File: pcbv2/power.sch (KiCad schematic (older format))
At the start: 13 parts, among them SW4 SW_SPDT, U2 AMS1117-3.3, U4 TPS610986DSET, U6 PMPB15XP,115

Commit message: feat(pcbv2): add part numbers to schematics
mostly LCSC / Digikey. Some components still missing, will
add them soon.
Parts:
- U6: Description (none) -> Trans MOSFET P-CH 12V 8.2A 6-Pin DFN-MD EP T/R; Field4 UDFN-6 Nexperia USA -> (none); Field5 Nexperia USA -> (none); Field6 None -> (none); Field7 Unavailable -> (none); Field8 Trans MOSFET P-CH 12V 8.2A 6-Pin DFN-MD EP T/R -> (none); LCSC Part (none) -> C294617
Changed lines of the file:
@@
 F 1 "PMPB15XP,115" H 4700 4700 50  0000 L CNN
 F 2 "PMPB15XP_115:MOSFET_PMPB55ENEAX" H 5350 5050 50  0001 L BNN
-F 3 "PMPB15XP,115" H 5350 5050 50  0001 L BNN
-F 4 "UDFN-6 Nexperia USA" H 5350 5050 50  0001 L BNN "Field4"
-F 5 "Nexperia USA" H 5350 5050 50  0001 L BNN "Field5"
-F 6 "None" H 5350 5050 50  0001 L BNN "Field6"
-F 7 "Unavailable" H 5350 5050 50  0001 L BNN "Field7"
-F 8 "Trans MOSFET P-CH 12V 8.2A 6-Pin DFN-MD EP T/R" H 5350 5050 50  0001 L BNN "Field8"
+F 3 "~" H 5350 5050 50  0001 L BNN
+F 4 "Trans MOSFET P-CH 12V 8.2A 6-Pin DFN-MD EP T/R" H 5350 5050 50  0001 L BNN "Description"
+F 5 "C294617" H 5350 5050 50  0001 C CNN "LCSC Part"
 	1    5350 5050
 	1    0    0    -1

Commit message: feat(pcbv2): add BOM part numbers
most parts there there, still missing a few
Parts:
- C12: LCSC Part (none) -> C27279; Vendor (none) -> TLJA107M006R0800
- L2: LCSC Part (none) -> C307785; Vendor (none) -> NLCV32T-4R7M-PFR
- R14: LCSC Part (none) -> C23151; Vendor (none) -> 0603WAF3900T5E
- SW4: Digikey Part (none) -> CKN9560-ND; Vendor (none) -> OS102011MA1QS1
- U2: LCSC Part (none) -> C6186
- U4: Digikey Part (none) -> 296-44974-1-ND; LCSC Part (none) -> C73820
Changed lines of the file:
@@
 F 2 "SON50P150X150X80-6N:SON50P150X150X80-6N" H 7400 3450 50  0001 C CNN
 F 3 "" H 7400 3450 50  0001 C CNN
+F 4 "296-44974-1-ND" H 7500 3600 50  0001 C CNN "Digikey Part"
+F 5 "C73820" H 7500 3600 50  0001 C CNN "LCSC Part"
 	1    7500 3600
 	1    0    0    -1
@@
 F 2 "Package_TO_SOT_SMD:SOT-223-3_TabPin2" H 4550 3700 50  0001 C CNN
 F 3 "http://www.advanced-monolithic.com/pdf/ds1117.pdf" H 4650 3250 50  0001 C CNN
+F 4 "C6186" H 4550 3500 50  0001 C CNN "LCSC Part"
 	1    4550 3500
 	1    0    0    -1
@@
 F 2 "Inductor_SMD:L_1210_3225Metric" H 6750 3600 50  0001 C CNN
 F 3 "~" H 6750 3600 50  0001 C CNN
+F 4 "C307785" H 6750 3600 50  0001 C CNN "LCSC Part"
+F 5 "NLCV32T-4R7M-PFR" H 6750 3600 50  0001 C CNN "Vendor"
 	1    6750 3600
 	1    0    0    -1
@@
 F 2 "Resistor_SMD:R_0603_1608Metric" V 6230 3750 50  0001 C CNN
 F 3 "~" H 6300 3750 50  0001 C CNN
+F 4 "C23151" H 6300 3750 50  0001 C CNN "LCSC Part"
+F 5 "0603WAF3900T5E" H 6300 3750 50  0001 C CNN "Vendor"
 	1    6300 3750
 	1    0    0    -1
@@
 F 2 "Button_Switch_THT:SW_CuK_OS102011MA1QN1_SPDT_Angled" H 5600 3600 50  0001 C CNN
 F 3 "" H 5600 3600 50  0001 C CNN
+F 4 "CKN9560-ND" H 5600 3600 50  0001 C CNN "Digikey Part"
+F 5 "OS102011MA1QS1" H 5600 3600 50  0001 C CNN "Vendor"
 	1    5600 3600
 	-1   0    0    1
@@
 F 2 "Capacitor_Tantalum_SMD:CP_EIA-3216-18_Kemet-A" H 6750 2950 50  0001 C CNN
 F 3 "~" H 6750 2950 50  0001 C CNN
+F 4 "C27279" H 6750 2950 50  0001 C CNN "LCSC Part"
+F 5 "TLJA107M006R0800" H 6750 2950 50  0001 C CNN "Vendor"
 	1    6750 2950
 	-1   0    0    1

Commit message: Added battery holders BOM data
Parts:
- BT1: footprint AA_battery_clip:BK-53_MPD_AAClip -> bcaaapc:bcaaapc; Digikey Part (none) -> BCAAAPC-ND
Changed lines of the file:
@@
 EESchema Schematic File Version 4
 LIBS:badge2-cache
-EELAYER 30 0
+EELAYER 26 0
 EELAYER END
 $Descr A4 11693 8268
@@
 F 0 "BT1" H 3768 4946 50  0000 L CNN
 F 1 "Battery_Cell" H 3768 4855 50  0000 L CNN
-F 2 "AA_battery_clip:BK-53_MPD_AAClip" V 3650 4910 50  0001 C CNN
-F 3 "~" V 3650 4910 50  0001 C CNN
+F 2 "bcaaapc:bcaaapc" V 3650 4910 50  0001 C CNN
+F 3 "http://www.memoryprotectiondevices.com/datasheets/BCAAAPC-datasheet.pdf" V 3650 4910 50  0001 C CNN
+F 4 "BCAAAPC-ND" H 3650 4850 50  0001 C CNN "Digikey Part"
 	1    3650 4850
 	0    1    1    0

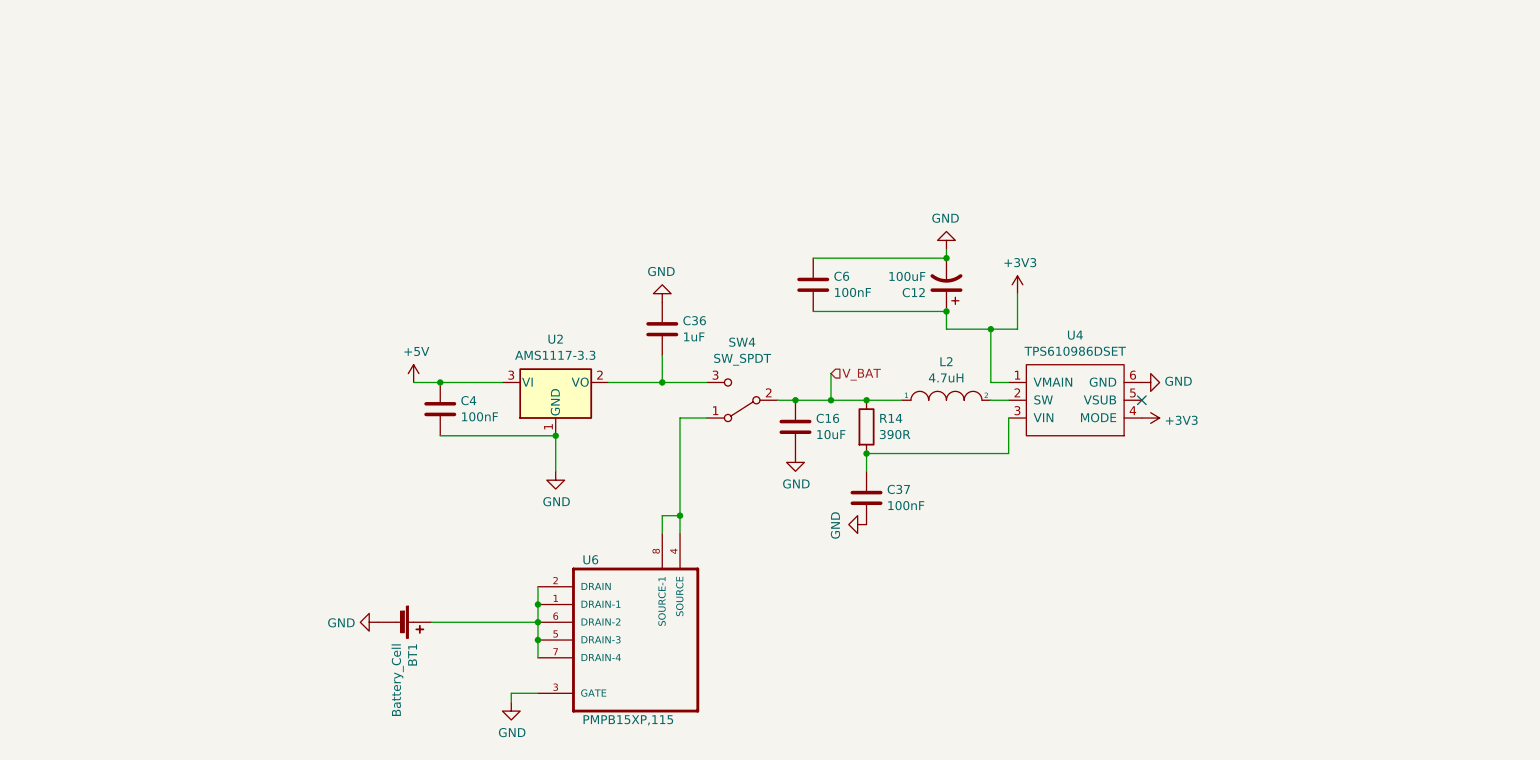
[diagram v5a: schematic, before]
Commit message: fix(pcbv2): remove AMS1117-3.3 regulator
We already have RT9013-33GB that does the same.
This also fixes an issue where the power switch would not be able to cut USB/LiPo power.
Also move LiPo circuit into power schematic.
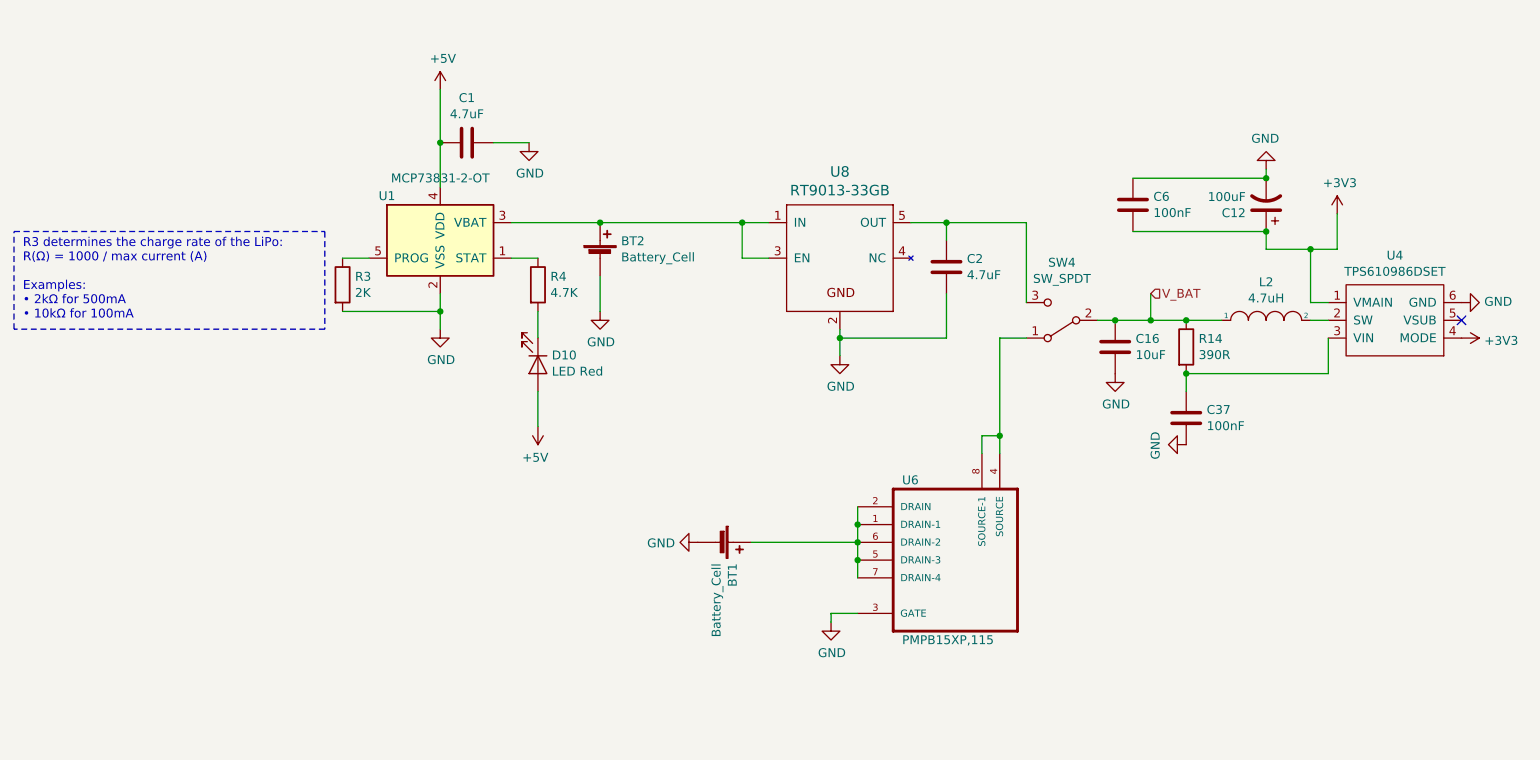
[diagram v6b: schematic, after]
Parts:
- removed C36: 1uF, Capacitor_SMD:C_0603_1608Metric, symbol Device:C
- removed C4: 100nF, Capacitor_SMD:C_0603_1608Metric, symbol Device:C
- removed U2: AMS1117-3.3, Package_TO_SOT_SMD:SOT-223-3_TabPin2, symbol Regulator_Linear:AMS1117-3.3
- added BT2: Battery_Cell, jst:JST_PH_B2B-PH-K_02x2.00mm_Straight, symbol Device:Battery_Cell
- added C1, C2: 4.7uF, Capacitor_SMD:C_0603_1608Metric, symbol Device:C
- added D10: LED Red, LED_SMD:LED_0603_1608Metric, symbol Device:LED
- added R3: 2K, Resistor_SMD:R_0603_1608Metric, symbol Device:R
- added R4: 4.7K, Resistor_SMD:R_0603_1608Metric, symbol Device:R
- added U1: MCP73831-2-OT, Package_TO_SOT_SMD:SOT-23-5, symbol Battery_Management:MCP73831-2-OT
- added U8: RT9013-33GB, Package_TO_SOT_SMD:SOT-23-5, symbol RT9013:RT9013-XXXB
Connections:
- net +5V: now also C1.2, D10.2 (A), U1.4 (VDD)
- net GND: now also BT2.2 (-), C1.1, C2.2, R3.2, U1.2 (VSS), U8.2 (GND)
- net at SW4.3 (C): now also C2.1, U8.5 (OUT)
- new net: R4.1, U1.1 (STAT)
- new net: BT2.1 (+), U1.3 (VBAT), U8.1 (IN), U8.3 (EN)
- new net: R3.1, U1.5 (PROG)
- new net: D10.1 (K), R4.2
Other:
- note added: "R3 determines the charge rate of the LiPo:\nR(Ω) = 1000 / max current (A) \n\nExamples:\n• 2kΩ for 500mA\n• 10kΩ for 100mA"
- moved on the sheet: BT1, C12, C16, C37, C6, L2, R14, SW4, U4, U6

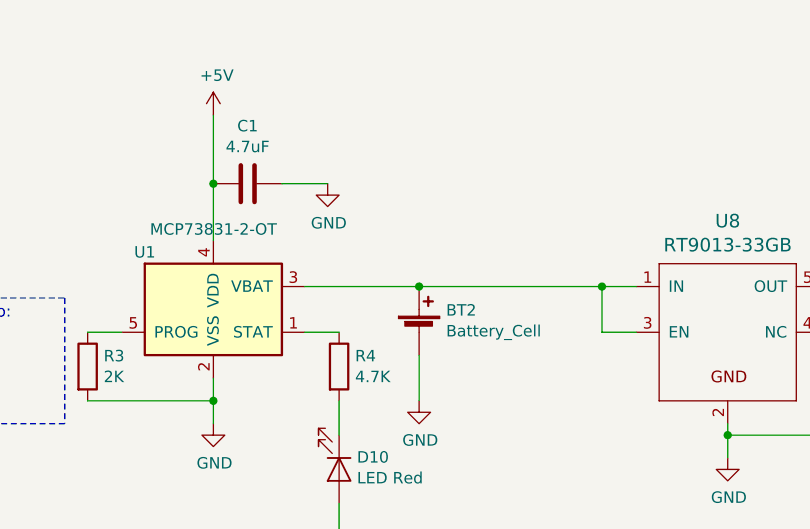
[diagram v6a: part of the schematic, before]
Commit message: feat(pcbv2): improve LiPo charging circuit
Add a transistor (Q3), that cuts the power from the LiPo when USB is connected,
allowing us to separate the battery from the rest of the circuit
while it's being charged.
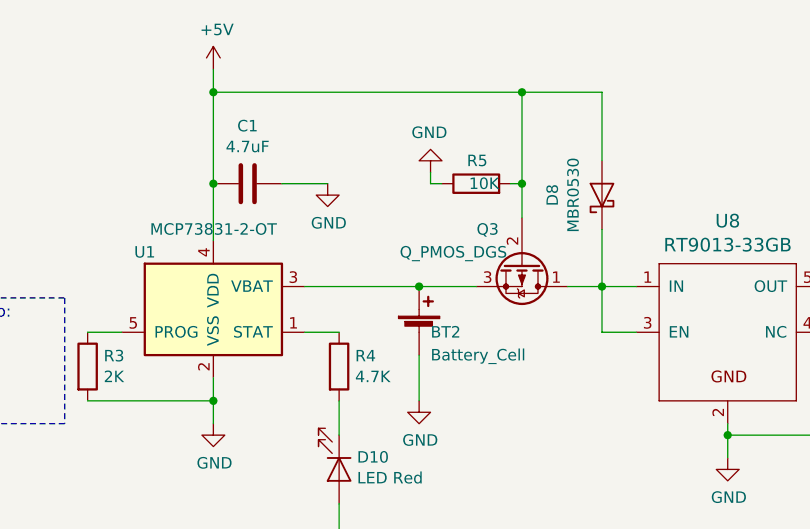
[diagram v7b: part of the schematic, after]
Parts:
- added D8: MBR0530, Diode_SMD:D_SOD-123, symbol Device:D_Schottky
- added Q3: Q_PMOS_DGS, Package_TO_SOT_SMD:SOT-23, symbol Device:Q_PMOS_DGS
- added R5: 10K, Resistor_SMD:R_0603_1608Metric, symbol Device:R
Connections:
- net +5V: now also D8.2 (A), Q3.2 (G), R5.2
- net GND: now also R5.1
- net at BT2.1 (+), U1.3 (VBAT): now also Q3.3 (S); no longer U8.1 (IN), U8.3 (EN)
- new net: D8.1 (K), Q3.1 (D), U8.1 (IN), U8.3 (EN)
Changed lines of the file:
@@
 L power:+5V #PWR0109
 U 1 1 5D9D5A8E
-P 3900 1850
-F 0 "#PWR0109" H 3900 1700 50  0001 C CNN
-F 1 "+5V" H 3915 2023 50  0000 C CNN
-F 2 "" H 3900 1850 50  0001 C CNN
-F 3 "" H 3900 1850 50  0001 C CNN
-	1    3900 1850
-	1    0    0    -1
-$EndComp
-Wire Wire Line
-	3900 1850 3900 2150
+P 3900 1650
+F 0 "#PWR0109" H 3900 1500 50  0001 C CNN
+F 1 "+5V" H 3915 1823 50  0000 C CNN
+F 2 "" H 3900 1650 50  0001 C CNN
+F 3 "" H 3900 1650 50  0001 C CNN
+	1    3900 1650
+	1    0    0    -1
+$EndComp
 Wire Wire Line
 	4300 2600 4800 2600
@@
 U 1 1 5D9D64A0
 P 4800 2800
-F 0 "BT2" H 4918 2896 50  0000 L CNN
-F 1 "Battery_Cell" H 4918 2805 50  0000 L CNN
+F 0 "BT2" H 4850 2800 50  0000 L CNN
+F 1 "Battery_Cell" H 4850 2700 50  0000 L CNN
 F 2 "jst:JST_PH_B2B-PH-K_02x2.00mm_Straight" V 4800 2860 50  0001 C CNN
 F 3 "http://www.jst-mfg.com/product/pdf/eng/ePH.pdf" V 4800 2860 50  0001 C CNN
@@
 	6750 3250 6150 3250
 Wire Wire Line
-	4800 2600 5600 2600
+	4800 2600 5050 2600
 Connection ~ 6150 3250
 Wire Wire Line
@@
 	7200 2600 6750 2600
 Connection ~ 6750 2600
+$Comp
+L Device:Q_PMOS_DGS Q3
+U 1 1 5DBF0489
+P 5250 2500
+F 0 "Q3" V 5100 2350 50  0000 C CNN
+F 1 "Q_PMOS_DGS" V 5200 2200 50  0000 C CNN
+F 2 "Package_TO_SOT_SMD:SOT-23" H 5450 2600 50  0001 C CNN
+F 3 "~" H 5250 2500 50  0001 C CNN
+F 4 "C15127" V 5250 2500 50  0001 C CNN "LCSC Part"
+F 5 "AO3401A" V 5250 2500 50  0001 C CNN "Vendor"
+	1    5250 2500
+	0    1    1    0
+$EndComp
+Wire Wire Line
+	5450 2600 5600 2600
+Wire Wire Line
+	3900 1650 3900 1750
+Wire Wire Line
+	5250 2300 5250 2150
+Connection ~ 3900 1750
+Wire Wire Line
+	3900 1750 3900 2150
+$Comp
+L Device:R R?
+U 1 1 5DBFE530
+P 5050 2150
+AR Path="/5DBFE530" Ref="R?"  Part="1"
+AR Path="/5C4AA0D1/5DBFE530" Ref="R5"  Part="1"
+F 0 "R5" V 5150 2100 50  0000 L CNN
+F 1 "10K" V 5050 2050 50  0000 L CNN
+F 2 "Resistor_SMD:R_0603_1608Metric" V 4980 2150 50  0001 C CNN
+F 3 "~" H 5050 2150 50  0001 C CNN
+F 4 "C25804" H 5050 2150 50  0001 C CNN "LCSC Part"
+F 5 "0603WAF1002T5E" H 5050 2150 50  0001 C CNN "Vendor"
+	1    5050 2150
+	0    -1   -1   0
+$EndComp
+Connection ~ 5250 2150
+Wire Wire Line
+	5250 2150 5250 1750
+$Comp
+L power:GND #PWR0113
+U 1 1 5DC02497
+P 4850 2100
+F 0 "#PWR0113" H 4850 1850 50  0001 C CNN
+F 1 "GND" H 4855 1927 50  0000 C CNN
+F 2 "" H 4850 2100 50  0001 C CNN
+F 3 "" H 4850 2100 50  0001 C CNN
+	1    4850 2100
+	-1   0    0    1
+$EndComp
+Wire Wire Line
+	4850 2150 4850 2100
+Wire Wire Line
+	3900 1750 5250 1750
+Connection ~ 5250 1750
+Wire Wire Line
+	5250 1750 5600 1750
+Wire Wire Line
+	5600 1750 5600 2050
+Wire Wire Line
+	5600 2350 5600 2600
+Wire Wire Line
+	4900 2150 4850 2150
+Wire Wire Line
+	5200 2150 5250 2150
+$Comp
+L Device:D_Schottky D8
+U 1 1 5DC18B11
+P 5600 2200
+F 0 "D8" H 5600 2416 50  0000 C CNN
+F 1 "MBR0530" H 5600 2325 50  0000 C CNN
+F 2 "Diode_SMD:D_SOD-123" H 5600 2200 50  0001 C CNN
+F 3 "~" H 5600 2200 50  0001 C CNN
+F 4 "C77336" H 5600 2200 50  0001 C CNN "LCSC Part"
+	1    5600 2200
+	0    -1   -1   0
+$EndComp
 $EndSCHEMATC

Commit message: fix(pcbv2): Q3 mosfet orientation
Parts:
- Q3: symbol Device:Q_PMOS_DGS -> Device:Q_PMOS_GSD
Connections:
- net +5V: now also Q3.1 (G); no longer Q3.2 (G)
- net at D8.1 (K), U8.1 (IN), U8.3 (EN): now also Q3.2 (S); no longer Q3.1 (D)
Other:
- moved on the sheet: BT2, D8, Q3, R5
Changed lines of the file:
@@
 	1    0    0    -1
 $EndComp
-Wire Wire Line
-	4300 2600 4800 2600
 $Comp
 L Device:Battery_Cell BT2
 U 1 1 5D9D64A0
-P 4800 2800
-F 0 "BT2" H 4850 2800 50  0000 L CNN
-F 1 "Battery_Cell" H 4850 2700 50  0000 L CNN
-F 2 "jst:JST_PH_B2B-PH-K_02x2.00mm_Straight" V 4800 2860 50  0001 C CNN
-F 3 "http://www.jst-mfg.com/product/pdf/eng/ePH.pdf" V 4800 2860 50  0001 C CNN
-F 4 "B2B-PH-K-S(LF)(SN)" H 4800 2800 50  0001 C CNN "Digikey Part"
-	1    4800 2800
-	1    0    0    -1
-$EndComp
-Wire Wire Line
-	4800 2900 4800 3100
+P 4850 2400
+F 0 "BT2" H 4850 2400 50  0000 L CNN
+F 1 "Battery_Cell" H 4650 2300 50  0000 L CNN
+F 2 "jst:JST_PH_B2B-PH-K_02x2.00mm_Straight" V 4850 2460 50  0001 C CNN
+F 3 "http://www.jst-mfg.com/product/pdf/eng/ePH.pdf" V 4850 2460 50  0001 C CNN
+F 4 "B2B-PH-K-S(LF)(SN)" H 4850 2400 50  0001 C CNN "Digikey Part"
+	1    4850 2400
+	-1   0    0    1
+$EndComp
 Connection ~ 3900 3100
 Wire Wire Line
@@
 $EndComp
 Wire Wire Line
-	4450 3550 4450 3750
+	4450 3550 4450 3650
 $Comp
 L RT9013:RT9013-XXXB U8
@@
 	1    0    0    -1
 $EndComp
-Connection ~ 4800 2600
 Wire Wire Line
 	5600 2600 5600 2800
@@
 Wire Wire Line
 	6750 3250 6150 3250
-Wire Wire Line
-	4800 2600 5050 2600
 Connection ~ 6150 3250
 Wire Wire Line
@@
 	7200 2600 6750 2600
 Connection ~ 6750 2600
-$Comp
-L Device:Q_PMOS_DGS Q3
-U 1 1 5DBF0489
-P 5250 2500
-F 0 "Q3" V 5100 2350 50  0000 C CNN
-F 1 "Q_PMOS_DGS" V 5200 2200 50  0000 C CNN
-F 2 "Package_TO_SOT_SMD:SOT-23" H 5450 2600 50  0001 C CNN
-F 3 "~" H 5250 2500 50  0001 C CNN
-F 4 "C15127" V 5250 2500 50  0001 C CNN "LCSC Part"
-F 5 "AO3401A" V 5250 2500 50  0001 C CNN "Vendor"
-	1    5250 2500
-	0    1    1    0
-$EndComp
 Wire Wire Line
 	5450 2600 5600 2600
-Wire Wire Line
-	3900 1650 3900 1750
-Wire Wire Line
-	5250 2300 5250 2150
-Connection ~ 3900 1750
-Wire Wire Line
-	3900 1750 3900 2150
 $Comp
 L Device:R R?
 U 1 1 5DBFE530
-P 5050 2150
+P 5050 3000
 AR Path="/5DBFE530" Ref="R?"  Part="1"
 AR Path="/5C4AA0D1/5DBFE530" Ref="R5"  Part="1"
-F 0 "R5" V 5150 2100 50  0000 L CNN
-F 1 "10K" V 5050 2050 50  0000 L CNN
-F 2 "Resistor_SMD:R_0603_1608Metric" V 4980 2150 50  0001 C CNN
-F 3 "~" H 5050 2150 50  0001 C CNN
-F 4 "C25804" H 5050 2150 50  0001 C CNN "LCSC Part"
-F 5 "0603WAF1002T5E" H 5050 2150 50  0001 C CNN "Vendor"
-	1    5050 2150
+F 0 "R5" V 5150 2950 50  0000 L CNN
+F 1 "10K" V 5050 2900 50  0000 L CNN
+F 2 "Resistor_SMD:R_0603_1608Metric" V 4980 3000 50  0001 C CNN
+F 3 "~" H 5050 3000 50  0001 C CNN
+F 4 "C25804" H 5050 3000 50  0001 C CNN "LCSC Part"
+F 5 "0603WAF1002T5E" H 5050 3000 50  0001 C CNN "Vendor"
+	1    5050 3000
 	0    -1   -1   0
 $EndComp
-Connection ~ 5250 2150
-Wire Wire Line
-	5250 2150 5250 1750
 $Comp
 L power:GND #PWR0113
 U 1 1 5DC02497
-P 4850 2100
-F 0 "#PWR0113" H 4850 1850 50  0001 C CNN
-F 1 "GND" H 4855 1927 50  0000 C CNN
-F 2 "" H 4850 2100 50  0001 C CNN
-F 3 "" H 4850 2100 50  0001 C CNN
-	1    4850 2100
+P 4850 2050
+F 0 "#PWR0113" H 4850 1800 50  0001 C CNN
+F 1 "GND" H 4855 1877 50  0000 C CNN
+F 2 "" H 4850 2050 50  0001 C CNN
+F 3 "" H 4850 2050 50  0001 C CNN
+	1    4850 2050
 	-1   0    0    1
 $EndComp
 Wire Wire Line
-	4850 2150 4850 2100
-Wire Wire Line
-	3900 1750 5250 1750
-Connection ~ 5250 1750
-Wire Wire Line
-	5250 1750 5600 1750
-Wire Wire Line
-	5600 1750 5600 2050
-Wire Wire Line
-	5600 2350 5600 2600
-Wire Wire Line
-	4900 2150 4850 2150
-Wire Wire Line
-	5200 2150 5250 2150
+	5200 3000 5250 3000
+$Comp
+L Device:Q_PMOS_GSD Q3
+U 1 1 5DBF0489
+P 5250 2700
+F 0 "Q3" V 5600 2700 50  0000 C CNN
+F 1 "Q_PMOS_DGS" V 5500 2700 50  0000 C CNN
+F 2 "Package_TO_SOT_SMD:SOT-23" H 5450 2800 50  0001 C CNN
+F 3 "~" H 5250 2700 50  0001 C CNN
+F 4 "C15127" V 5250 2700 50  0001 C CNN "LCSC Part"
+F 5 "AO3401A" V 5250 2700 50  0001 C CNN "Vendor"
+	1    5250 2700
+	0    -1   -1   0
+$EndComp
+Wire Wire Line
+	4450 3650 5250 3650
+Wire Wire Line
+	5250 3650 5250 3250
+Connection ~ 4450 3650
+Wire Wire Line
+	4450 3650 4450 3750
+Wire Wire Line
+	5600 2800 5600 2950
+Connection ~ 5600 2800
+Wire Wire Line
+	5600 3250 5250 3250
+Connection ~ 5250 3250
+Wire Wire Line
+	5250 3250 5250 3000
+Wire Wire Line
+	3900 1650 3900 2150
+Wire Wire Line
+	4300 2600 4850 2600
+Connection ~ 4850 2600
+Wire Wire Line
+	4850 2600 5050 2600
+Connection ~ 5250 3000
+Wire Wire Line
+	5250 3000 5250 2900
+Wire Wire Line
+	4850 2300 4850 2050
+Wire Wire Line
+	4800 3000 4800 3100
+Wire Wire Line
+	4800 3000 4900 3000
 $Comp
 L Device:D_Schottky D8
 U 1 1 5DC18B11
-P 5600 2200
-F 0 "D8" H 5600 2416 50  0000 C CNN
-F 1 "MBR0530" H 5600 2325 50  0000 C CNN
-F 2 "Diode_SMD:D_SOD-123" H 5600 2200 50  0001 C CNN
-F 3 "~" H 5600 2200 50  0001 C CNN
-F 4 "C77336" H 5600 2200 50  0001 C CNN "LCSC Part"
-	1    5600 2200
-	0    -1   -1   0
+P 5600 3100
+F 0 "D8" H 5600 3000 50  0000 C CNN
+F 1 "MBR0530" H 5600 3225 50  0000 C CNN
+F 2 "Diode_SMD:D_SOD-123" H 5600 3100 50  0001 C CNN
+F 3 "~" H 5600 3100 50  0001 C CNN
+F 4 "C77336" H 5600 3100 50  0001 C CNN "LCSC Part"
+	1    5600 3100
+	0    1    1    0
 $EndComp
 $EndSCHEMATC
